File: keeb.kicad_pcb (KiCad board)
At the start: 2 copper layers, 266.7 x 98.7 mm, 156 parts, among them J1 AudioJack3, J101 USB_C_Receptacle_USB2.0, J102 AVR-ISP-6, SW101 SW_Push, SW102 SW_Push, SW103 SW_Push, SW104 SW_Push, SW105 SW_Push, SW106 SW_Push, SW107 SW_Push, SW108 SW_Push, SW109 SW_Push, SW110 SW_Push, SW111 SW_Push, SW112 SW_Push, SW113 SW_Push, SW114 SW_Push, SW115 SW_Push, SW116 SW_Push, SW117 SW_Push, SW118 SW_Push, SW119 SW_Push, SW120 SW_Push, SW121 SW_Push, SW122 SW_Push, SW123 SW_Push, SW124 SW_Push, SW125 SW_Push, SW126 SW_Push, SW127 SW_Push, SW128 SW_Push, SW129 SW_Push, SW130 SW_Push, SW131 SW_Push, SW132 SW_Push, SW133 SW_Push, SW134 SW_Push, SW135 SW_Push, SW136 SW_Push, SW137 SW_Push, SW138 SW_Push, SW139 SW_Push, SW140 SW_Push, SW141 SW_Push, SW142 SW_Push, SW143 SW_Push, SW144 SW_Push, SW145 SW_Push, SW146 SW_Push, SW147 SW_Push, SW148 SW_Push, SW149 SW_Push, SW150 SW_Push, SW151 SW_Push, SW152 SW_Push, SW153 SW_Push, SW154 SW_Push, SW155 SW_Push, SW156 SW_Push, SW157 SW_Push, SW158 SW_Push, SW159 SW_Push, SW160 SW_Push, SW161 SW_Push, SW162 SW_Push, SW163 SW_Push, SW164 SW_Push, SW165 SW_Push, SW166 SW_Push, U102 ATmega32U4-AU, Y1 16Mhz

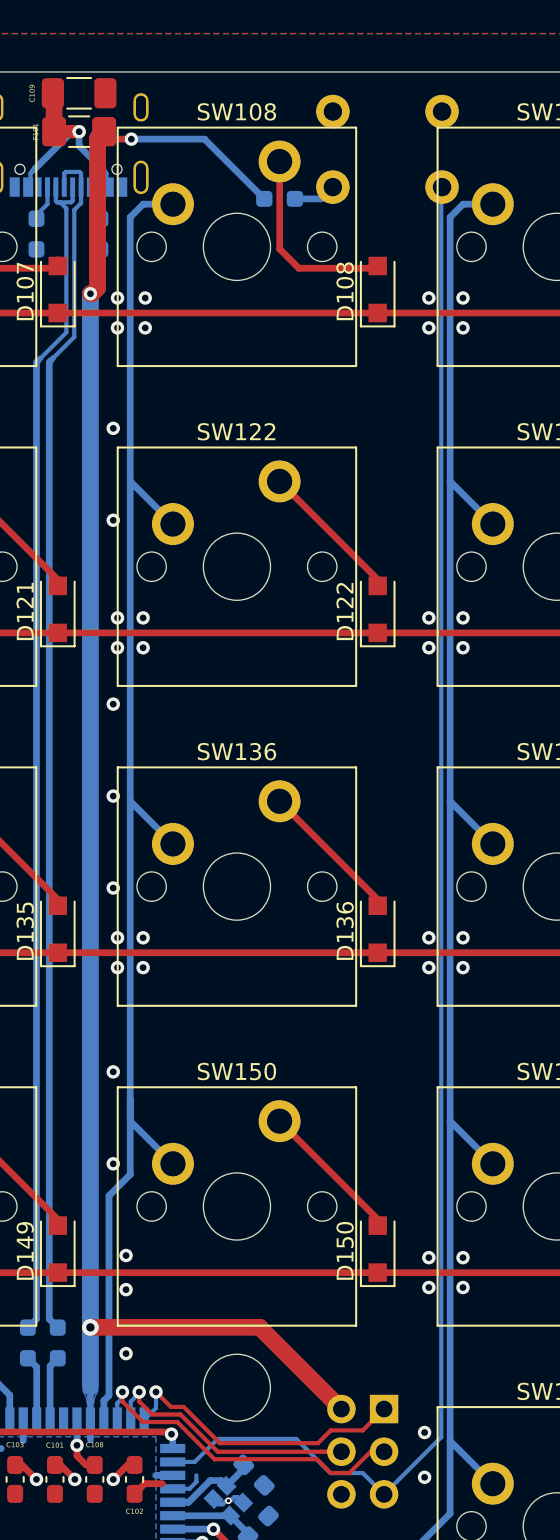
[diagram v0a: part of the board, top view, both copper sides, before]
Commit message: lp rst sw
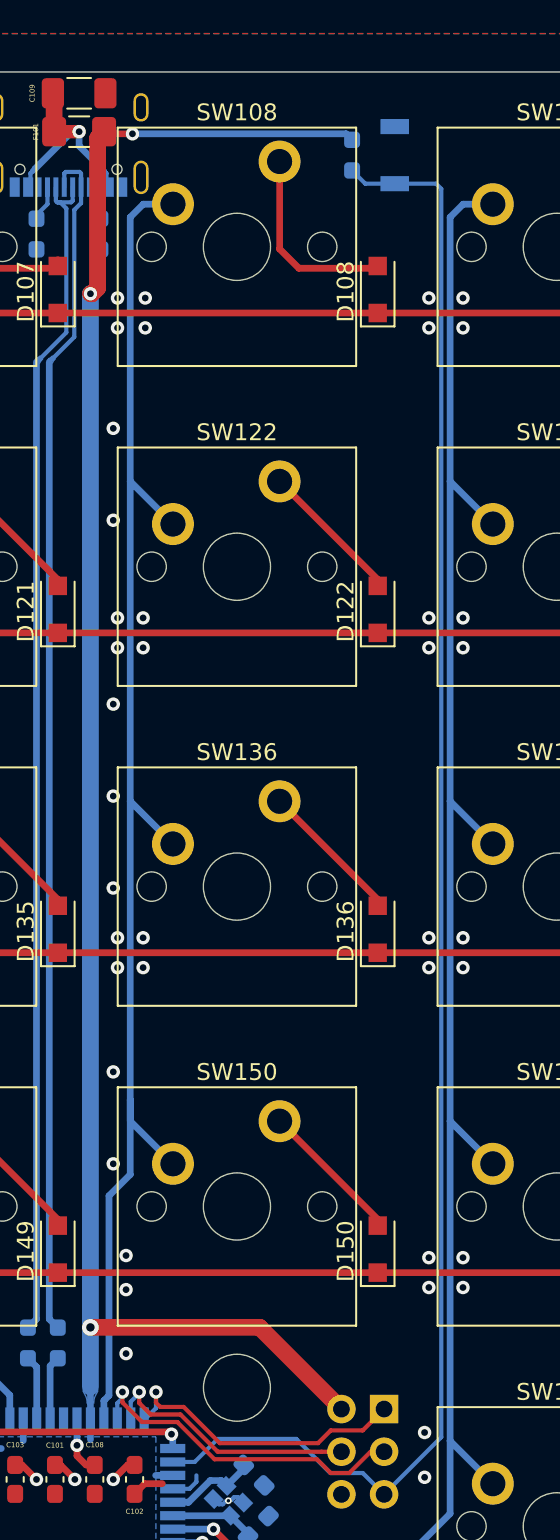
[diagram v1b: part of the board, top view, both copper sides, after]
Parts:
- RESET: footprint Button_Switch_THT:SW_PUSH_6mm_H5mm -> Button_Switch_SMD:SW_SPST_B3U-1000P
- moved R105 5.04 mm to (226.6, 115.2), turned to 90 degrees
- moved RESET 4.15 mm to (229.1, 115.2), turned to 90 degrees
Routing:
- net +5V: track 120.1 -> 123.9 mm
- net ~RESET: track 96.2 -> 99.4 mm
